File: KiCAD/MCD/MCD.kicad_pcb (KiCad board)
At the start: 2 copper layers, 196.5 x 115 mm, 76 parts, among them J1 DBUS_LOW, J2 DBUS_HIGH, J3 ABUS, J4 POWER, J5 JTAG, J6 Conn_01x02_Male, J7 DUART A, J8 DUART B, SW1 SW_Push, U1 XC9572XL-10VQG44C, U10 STM1001LWX6F, U2 AS6C1008-55PCN, U3 AS6C1008-55PCN, U4 SST39SF020A-70-4C-PHE, U5 SST39SF020A-70-4C-PHE, U6 XR68C681CJ-F, U7 AP2114HA-3.3TRG1, U8 MAX6816EUS_T, U9 MC68000FN, Y1 ECS-100AX-036, Y2 ECS-100AX-080

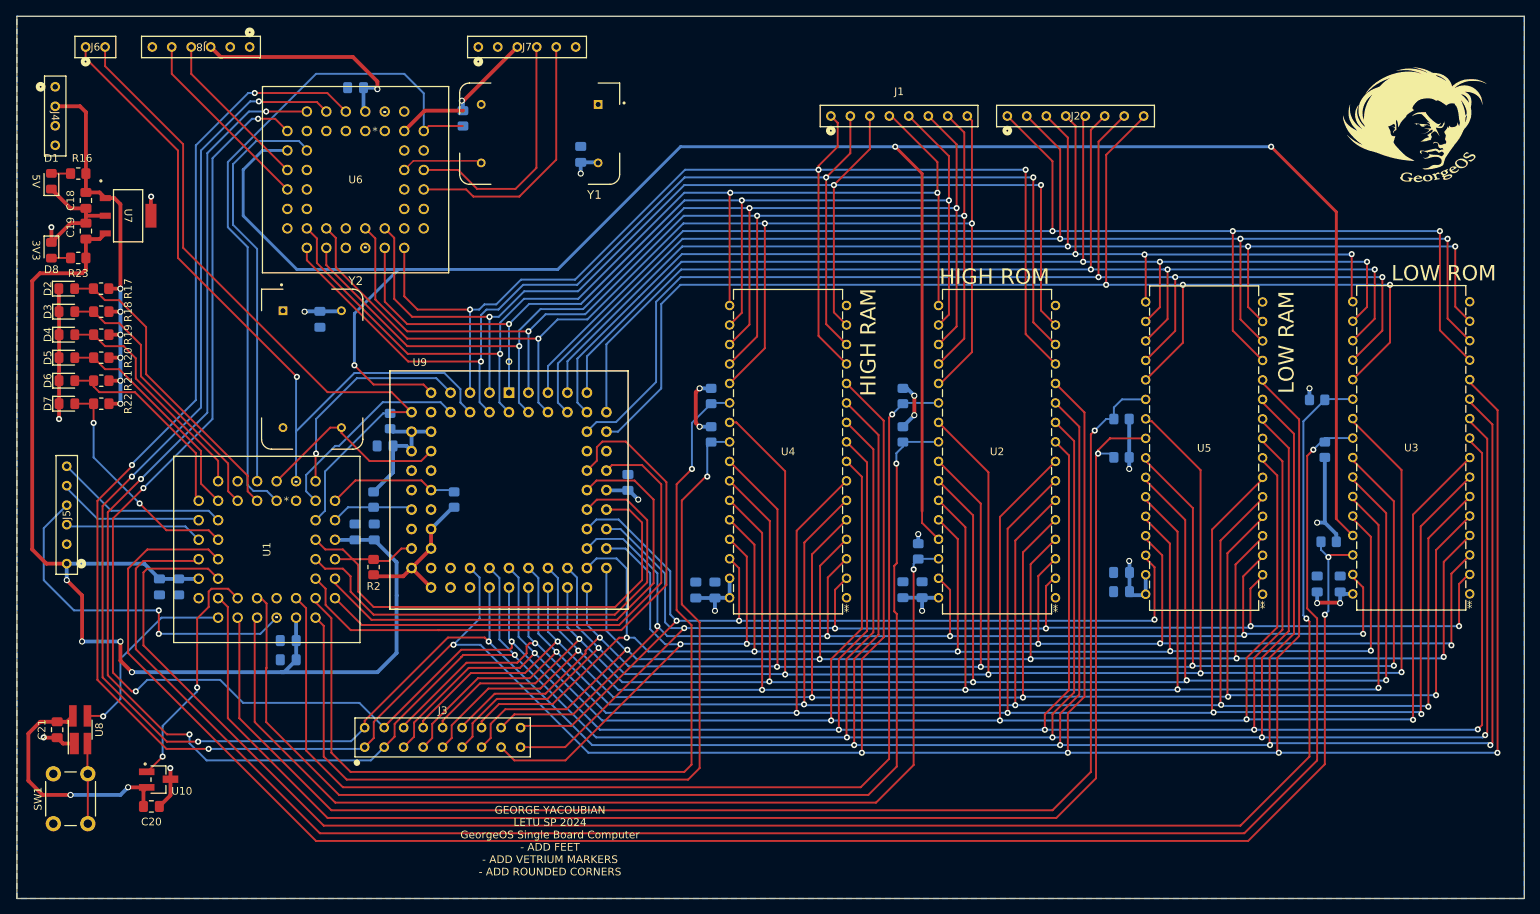
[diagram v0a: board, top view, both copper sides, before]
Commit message: FINISHED!!! (I THINK)
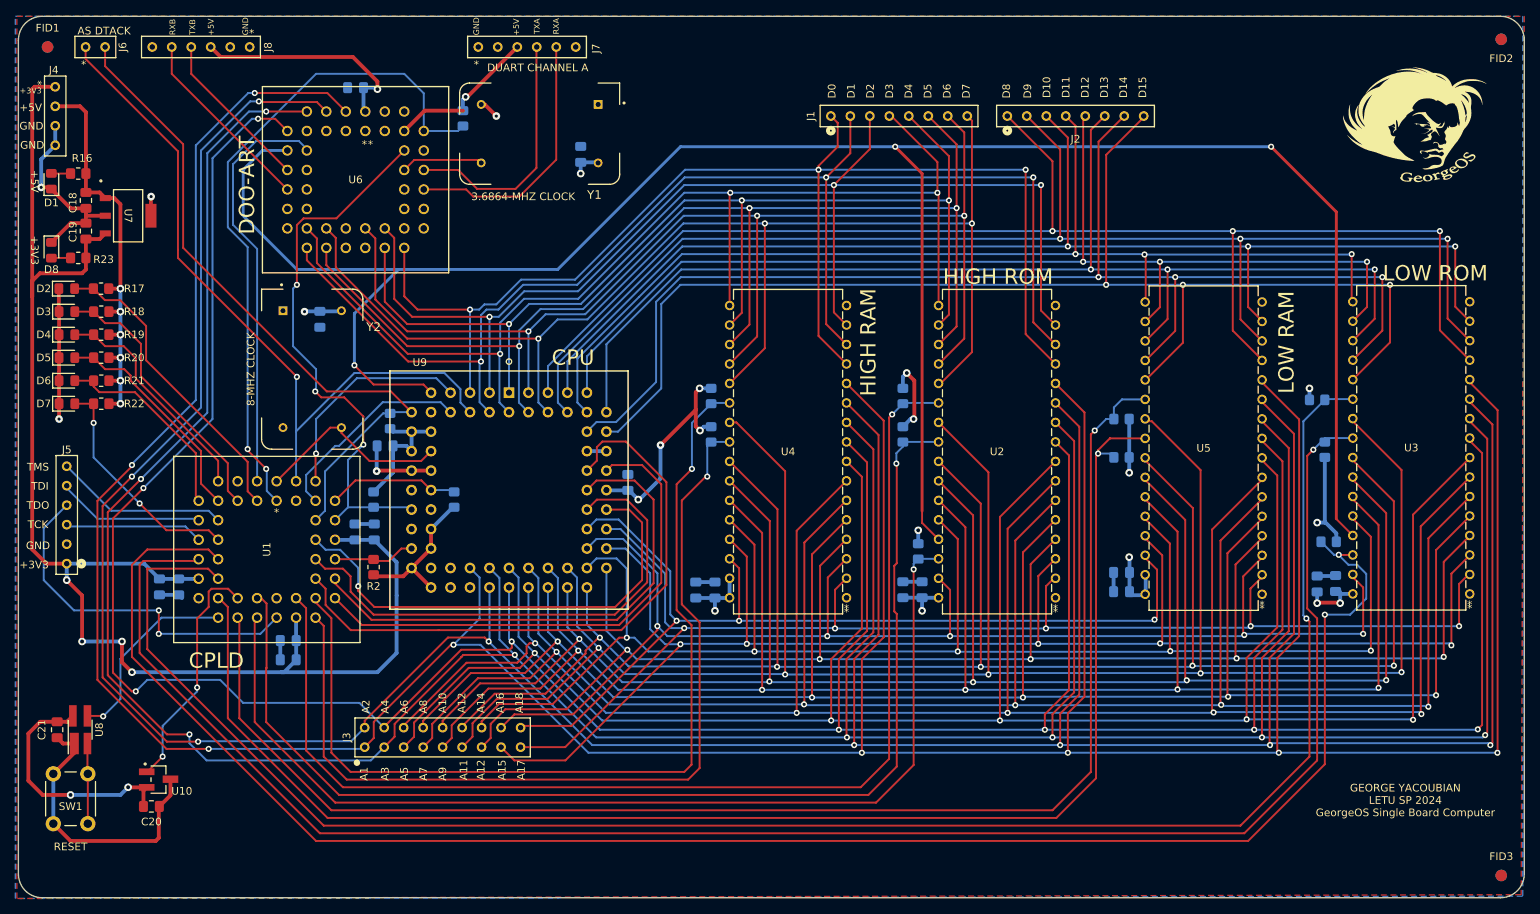
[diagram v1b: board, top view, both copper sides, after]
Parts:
- added FID1: Fiducial, Fiducial:Fiducial_1.5mm_Mask3mm, F.Cu at (104.5, 75.5)
- added FID2: Fiducial, Fiducial:Fiducial_1.5mm_Mask3mm, F.Cu at (294.0, 74.5)
- added FID3: Fiducial, Fiducial:Fiducial_1.5mm_Mask3mm, F.Cu at (294.0, 183.5)
- added FID4: Fiducial, Fiducial:Fiducial_1.5mm_Mask3mm, B.Cu at (104.5, 75.5)
- added FID5: Fiducial, Fiducial:Fiducial_1.5mm_Mask3mm, B.Cu at (294.0, 183.5)
- added FID6: Fiducial, Fiducial:Fiducial_1.5mm_Mask3mm, B.Cu at (294.0, 74.5)
- moved C2 0.60 mm to (272.4, 145.4)
- moved U5 0.07 mm to (262.8, 146.8)
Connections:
- D1 pad 2: /3V3_LED -> /5V_LED
- R16 pad 2: /3V3_LED -> /5V_LED
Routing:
- net GND: track 47.9 -> 117.1 mm
- net RESET: track 10.8 -> 72.3 mm, vias 0 -> 3
- net +3V3: track 158.0 -> 188.2 mm
- net +5V: track 256.1 -> 277.0 mm, vias 26 -> 27
- net RAMHCE2: track 227.5 -> 232.7 mm
- net /5V_LED: track 0.00 -> 2.51 mm
- net /3V3_LED: track 5.02 -> 2.51 mm
- net DUARTCS: track 89.4 -> 88.4 mm, vias 0 -> 2
- net D14: track 165.9 -> 165.4 mm
- net D13: track 155.3 -> 154.8 mm
- net A19: track 62.6 -> 62.3 mm, vias 0 -> 1
- added copper zone on F.Cu, net +5V
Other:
- board size 196.5 x 115 mm -> 196.3 x 114.9 mm
- board text added: "+3V3"
- board text added: "+5V"
- board text added: "3.6864-MHZ CLOCK"
- board text added: "8-MHZ CLOCK"
- board text added: "A1"
- board text added: "A10"
- board text added: "A11"
- board text added: "A12"
- board text added: "A14"
- board text added: "A15"
- board text added: "A16"
- board text added: "A17"
- board text added: "A18"
- board text added: "A2"
- board text added: "A3"
- board text added: "A4"
- board text added: "A5"
- board text added: "A6"
- board text added: "A7"
- board text added: "A8"
- board text added: "A9"
- board text added: "AS"
- board text added: "CPLD"
- board text added: "CPU"
- board text added: "D0"
- board text added: "D1"
- board text added: "D10"
- board text added: "D11"
- board text added: "D12"
- board text added: "D13"
- board text added: "D14"
- board text added: "D15"
- board text added: "D2"
- board text added: "D3"
- board text added: "D4"
- board text added: "D5"
- board text added: "D6"
- board text added: "D7"
- board text added: "D8"
- board text added: "D9"
- board text added: "DOO-ART"
- board text added: "DTACK"
- board text added: "DUART CHANNEL A"
- board text added: "GEORGE YACOUBIAN LETU SP 2024 GeorgeOS Single Board Computer"
- board text added: "GND"
- board text added: "RESET"
- board text added: "RXA"
- board text added: "RXB"
- board text added: "TCK"
- board text added: "TDI"
- board text added: "TDO"
- board text added: "TMS"
- board text added: "TXA"
- board text added: "TXB"
- board text removed: "3V3"
- board text removed: "5V"
- board text removed: "GEORGE YACOUBIAN LETU SP 2024 GeorgeOS Single Board Computer - ADD FEET - ADD VETRIUM MARKERS - ADD ROUNDED CORNERS"
